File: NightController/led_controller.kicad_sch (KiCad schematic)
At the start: 54 parts, among them U1 EAST1410RGBW02, U401 LP5036

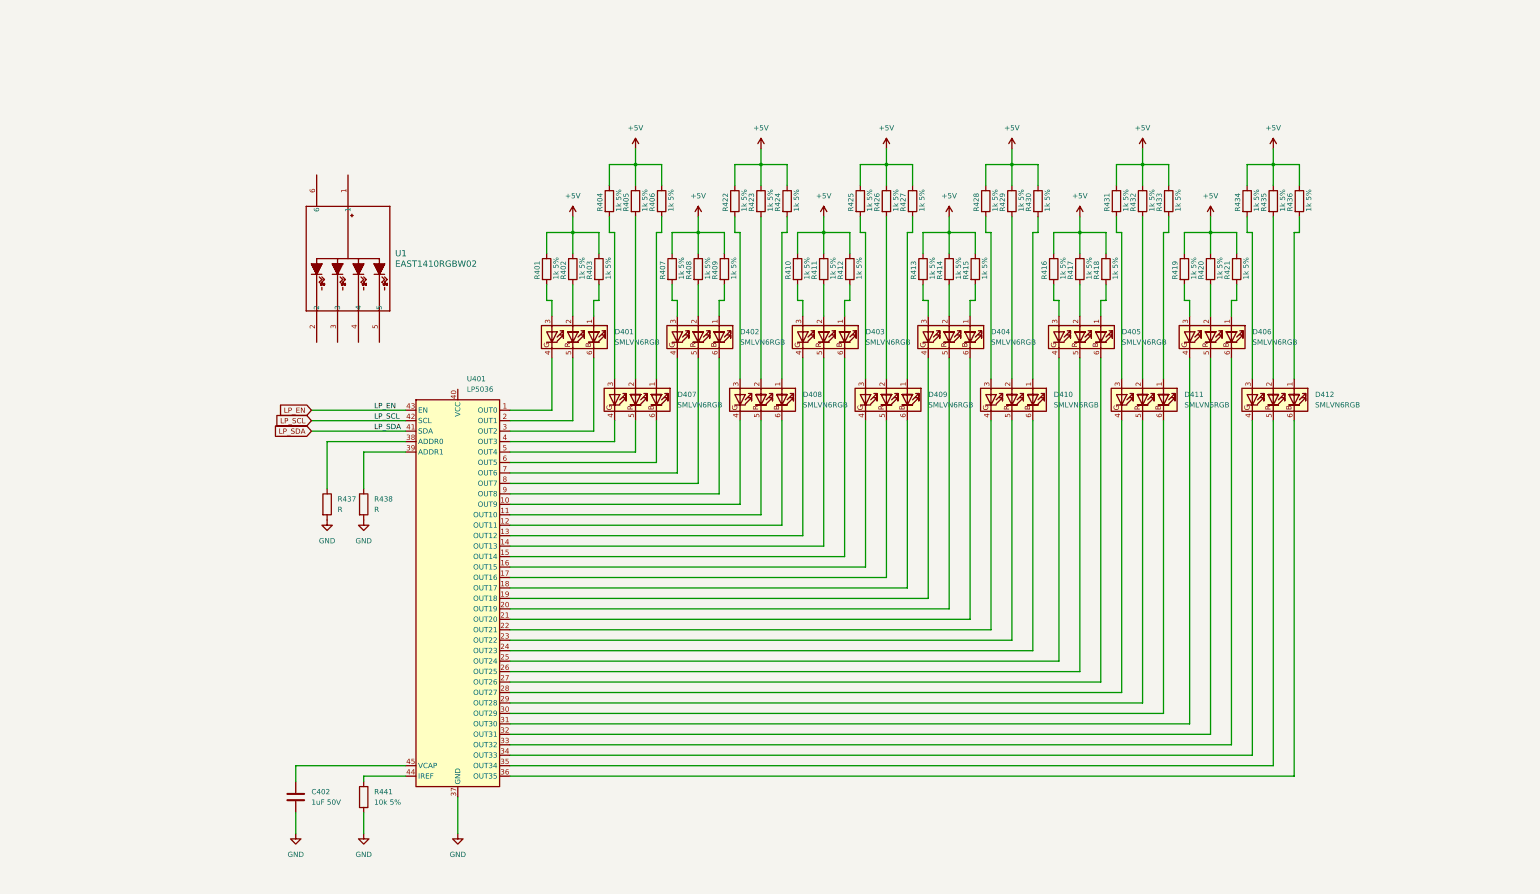
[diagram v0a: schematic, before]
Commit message: Working on files
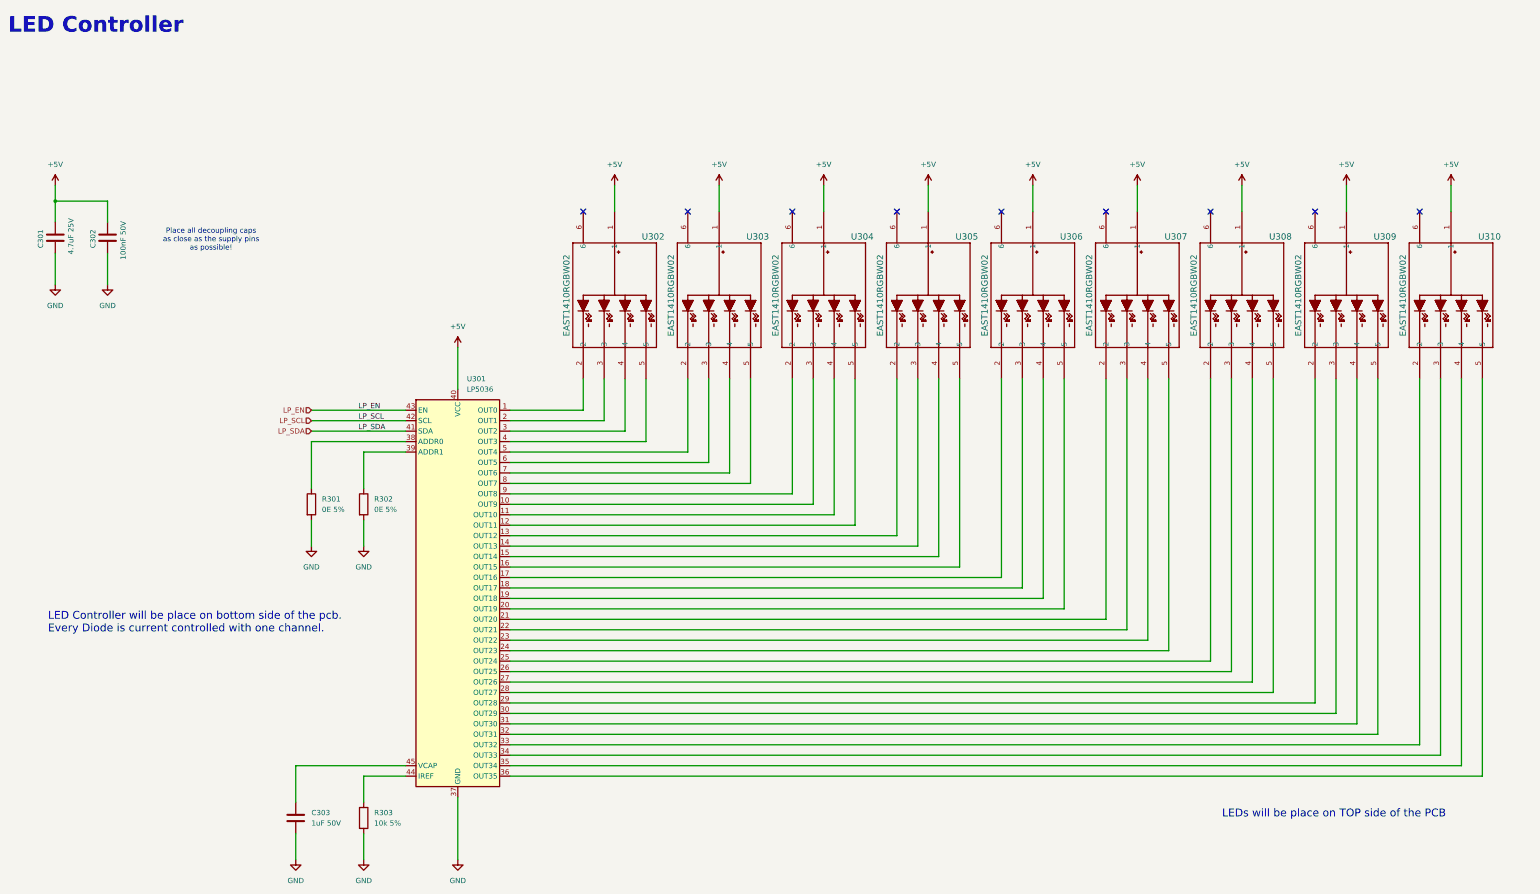
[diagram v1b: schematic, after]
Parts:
- removed D401, D402, D403, D404, D405, D406, D407, D408, D409, D410, D411, D412: SMLVN6RGB, LED_SMD:LED_ROHM_SMLVN6, symbol LED:SMLVN6RGB
- removed R401, R402, R403, R404, R405, R406, R407, R408, R409, R410, R411, R412, R413, R414, R415, R416, R417, R418, R419, R420, R421, R422, R423, R424, R425, R426, R427, R428, R429, R430, R431, R432, R433, R434, R435, R436: 1k 5%, symbol Device:R
- added C301: 4.7uF 25V, symbol Device:C
- added C302: 100nF 50V, symbol Device:C
- added U303, U304, U305, U306, U307, U308, U309, U310: EAST1410RGBW02, SMD_EAST1410RGBW02_EVE, symbol EAST1410RGBW02:EAST1410RGBW02
- R301: renamed from R437; value R -> 0E 5%
- R302: renamed from R438; value R -> 0E 5%
- renumbered C402 to C303, R441 to R303, U401 to U301, U1 to U302
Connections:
- net +5V: now also U301.40 (VCC), U302.1, C301.1, C302.1, U303.1, U304.1, U305.1, U306.1, U307.1, U308.1, U309.1, U310.1
- net GND: now also C301.2, C302.2
- net at U301.7 (OUT6): now also U303.4
- net at U301.8 (OUT7): now also U303.5
- net at U301.9 (OUT8): now also U304.2
- net at U301.28 (OUT27): now also U308.5
- net at U301.29 (OUT28): now also U309.2
- net at U301.30 (OUT29): now also U309.3
- net at U301.16 (OUT15): now also U305.5
- net at U301.17 (OUT16): now also U306.2
- net at U301.18 (OUT17): now also U306.3
- net at U301.34 (OUT33): now also U310.3
- net at U301.35 (OUT34): now also U310.4
- net at U301.36 (OUT35): now also U310.5
- net at U301.25 (OUT24): now also U308.2
- net at U301.26 (OUT25): now also U308.3
- net at U301.27 (OUT26): now also U308.4
- net at U301.10 (OUT9): now also U304.3
- net at U301.11 (OUT10): now also U304.4
- net at U301.12 (OUT11): now also U304.5
- net at U301.1 (OUT0): now also U302.2
- net at U301.13 (OUT12): now also U305.2
- net at U301.14 (OUT13): now also U305.3
- net at U301.15 (OUT14): now also U305.4
- net at U301.19 (OUT18): now also U306.4
- net at U301.2 (OUT1): now also U302.3
- net at U301.20 (OUT19): now also U306.5
- net at U301.21 (OUT20): now also U307.2
- net at U301.22 (OUT21): now also U307.3
- net at U301.23 (OUT22): now also U307.4
- net at U301.24 (OUT23): now also U307.5
- net at U301.3 (OUT2): now also U302.4
- net at U301.31 (OUT30): now also U309.4
- net at U301.32 (OUT31): now also U309.5
- net at U301.33 (OUT32): now also U310.2
- net at U301.4 (OUT3): now also U302.5
- net at U301.5 (OUT4): now also U303.2
- net at U301.6 (OUT5): now also U303.3
- no-connect marks 0 -> 9
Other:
- note added: "LED Controller"
- note added: "LED Controller will be place on bottom side of the pcb. Every Diode is current controlled with one channel."
- note added: "LEDs will be place on TOP side of the PCB"
- note added: "Place all decoupling caps as close as the supply pins as possible!"
- title: (none) -> NightLight
- moved on the sheet: C303, R301, R303, U302
